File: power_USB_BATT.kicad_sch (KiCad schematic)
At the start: 17 parts, among them IC1 MCP73834T-FCI_UN, IC2 AP2112M-3.3TRG1, Q1 MCQ9435-TP

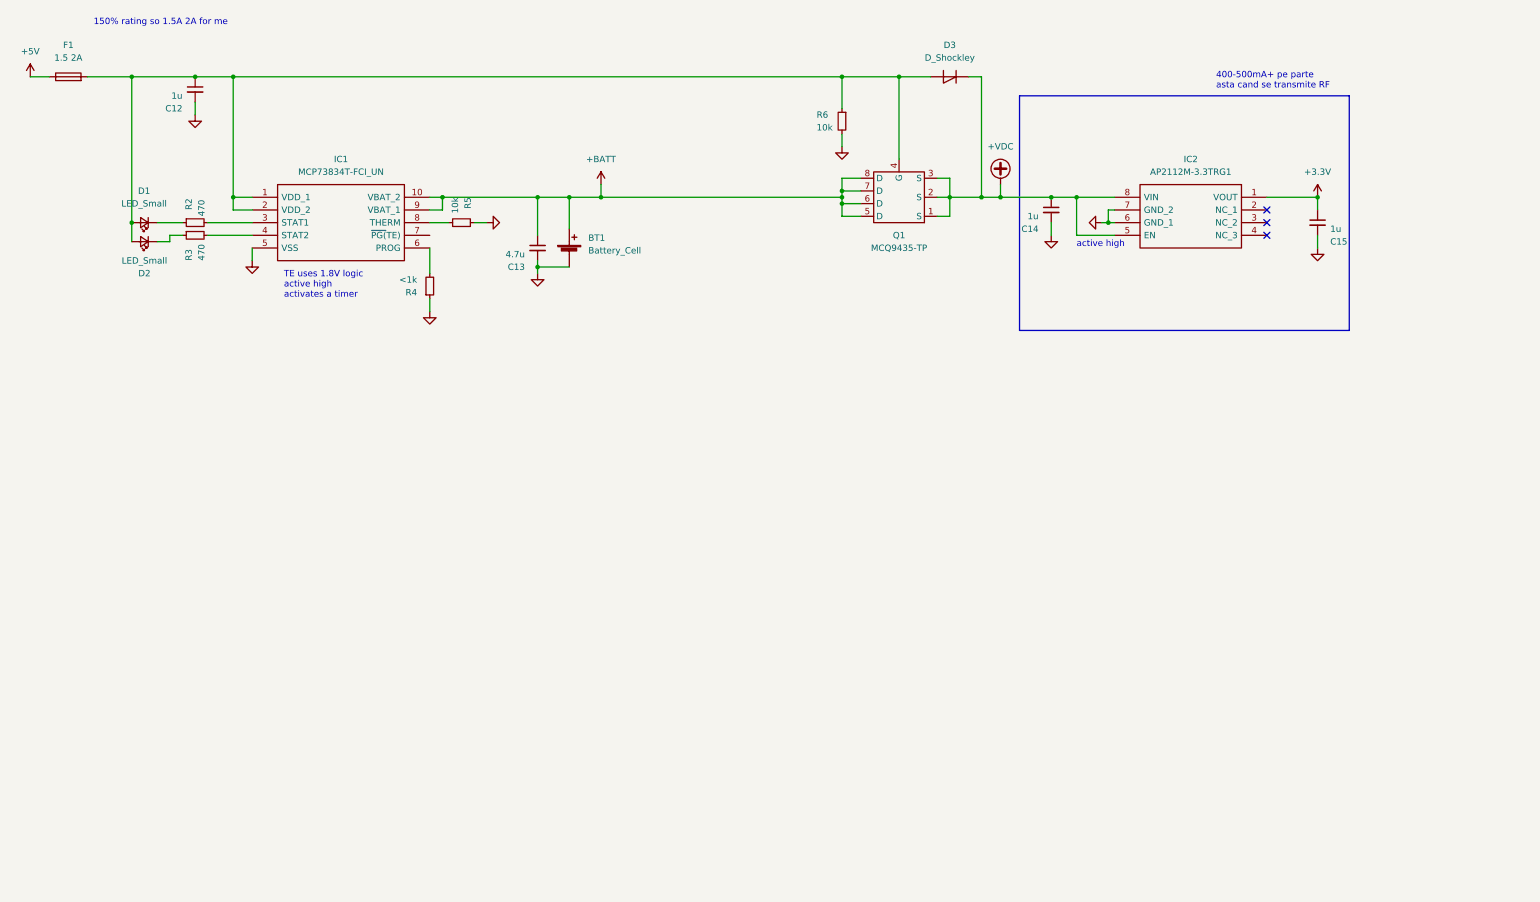
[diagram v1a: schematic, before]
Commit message: k
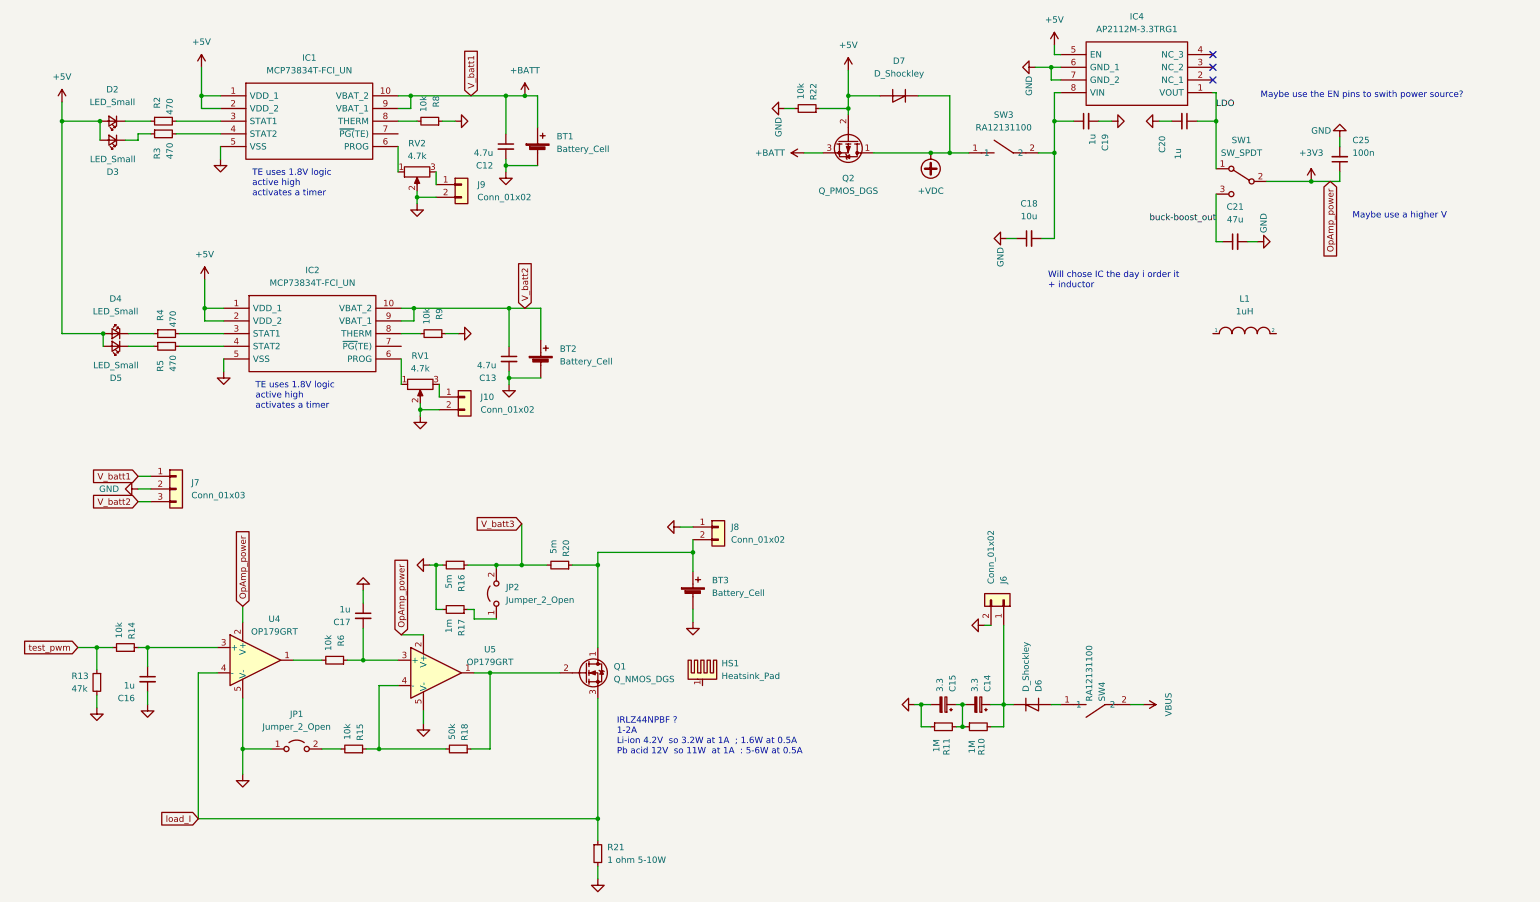
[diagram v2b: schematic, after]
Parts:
- removed C14, C15: 1u, symbol Device:C_Small
- removed D1: LED_Small, symbol Device:LED_Small
- removed D3: D_Shockley, Diode_THT:D_DO-15_P15.24mm_Horizontal, symbol Device:D_Shockley
- removed F1: 1.5 2A, symbol Device:Fuse
- removed IC2: AP2112M-3.3TRG1, SOIC127P600X170-8N, symbol SamacSys_Parts:AP2112M-3.3TRG1
- removed Q1: MCQ9435-TP, Package_SO:SOP-8_3.76x4.96mm_P1.27mm, symbol My_custom_lib:MCQ9435-TP
- added BT2, BT3: Battery_Cell, Connector_PinHeader_2.54mm:PinHeader_1x02_P2.54mm_Vertical, symbol Device:Battery_Cell
- added C14, C15: 3.3, Capacitor_THT:CP_Radial_D8.0mm_P3.50mm, symbol Device:C_Polarized_Small
- added C16, C17, C19, C20: 1u, Capacitor_SMD:C_0603_1608Metric_Pad1.08x0.95mm_HandSolder, symbol Device:C_Small
- added C18: 10u, symbol Device:C_Small
- added C21: 47u, symbol Device:C_Small
- added C25: 100n, Capacitor_SMD:C_0603_1608Metric_Pad1.08x0.95mm_HandSolder, symbol Device:C_Small
- added D3, D4, D5: LED_Small, LED_SMD:LED_0603_1608Metric_Pad1.05x0.95mm_HandSolder, symbol Device:LED_Small
- added D6, D7: D_Shockley, Diode_THT:D_A-405_P12.70mm_Horizontal, symbol Device:D_Shockley
- added HS1: Heatsink_Pad, symbol Mechanical:Heatsink_Pad
- added IC2: MCP73834T-FCI_UN, SamacSys_Parts:SOP50P490X110-10N, symbol SamacSys_Parts:MCP73834T-FCI_UN
- added IC4: AP2112M-3.3TRG1, SOIC127P600X170-8N, symbol SamacSys_Parts:AP2112M-3.3TRG1
- added J10, J9: Conn_01x02, Connector_PinHeader_2.54mm:PinHeader_1x02_P2.54mm_Vertical, symbol Connector_Generic:Conn_01x02
- added J6: Conn_01x02, Resistor_THT:R_Axial_DIN0309_L9.0mm_D3.2mm_P5.08mm_Vertical, symbol Connector_Generic:Conn_01x02
- added J7: Conn_01x03, Connector_PinHeader_2.54mm:PinHeader_1x03_P2.54mm_Vertical, symbol Connector_Generic:Conn_01x03
- added J8: Conn_01x02, Connector_Wago:Wago_734-132_1x02_P3.50mm_Vertical, symbol Connector_Generic:Conn_01x02
- added JP1, JP2: Jumper_2_Open, symbol Jumper:Jumper_2_Open
- added L1: 1uH, symbol pspice:INDUCTOR
- added Q1: Q_NMOS_DGS, symbol Device:Q_NMOS_DGS
- added Q2: Q_PMOS_DGS, symbol Device:Q_PMOS_DGS
- added R10, R11: 1M, Resistor_THT:R_Axial_DIN0411_L9.9mm_D3.6mm_P7.62mm_Vertical, symbol Device:R_Small
- added R13: 47k, Resistor_SMD:R_0603_1608Metric_Pad0.98x0.95mm_HandSolder, symbol Device:R_Small
- added R14, R15, R22, R8, R9: 10k, Resistor_SMD:R_0603_1608Metric_Pad0.98x0.95mm_HandSolder, symbol Device:R_Small
- added R16, R20: 5m, Resistor_SMD:R_0603_1608Metric_Pad0.98x0.95mm_HandSolder, symbol Device:R_Small
- added R17: 1m, Resistor_SMD:R_0603_1608Metric_Pad0.98x0.95mm_HandSolder, symbol Device:R_Small
- added R18: 50k, Resistor_SMD:R_0603_1608Metric_Pad0.98x0.95mm_HandSolder, symbol Device:R_Small
- added R21: 1 ohm 5-10W, symbol Device:R_Small
- added RV1, RV2: 4.7k, Z_mycustom_footprint_lib:2002102255, symbol Device:R_Potentiometer
- added SW1: SW_SPDT, symbol Switch:SW_SPDT
- added SW3, SW4: RA12131100, symbol My_custom_lib:RA12131100
- added U4, U5: OP179GRT, Package_TO_SOT_SMD:SOT-23-5, symbol Amplifier_Operational:OP179GRT
- BT1: footprint (none) -> Connector_PinHeader_2.54mm:PinHeader_1x02_P2.54mm_Vertical
- C12: value 1u -> 4.7u; footprint (none) -> Capacitor_SMD:C_0603_1608Metric_Pad1.08x0.95mm_HandSolder
- C13: footprint (none) -> Capacitor_SMD:C_0603_1608Metric_Pad1.08x0.95mm_HandSolder
- D2: footprint (none) -> LED_SMD:LED_0603_1608Metric_Pad1.05x0.95mm_HandSolder
- IC1: footprint SOP50P490X110-10N -> SamacSys_Parts:SOP50P490X110-10N
- R2, R3, R6: footprint (none) -> Resistor_SMD:R_0603_1608Metric_Pad0.98x0.95mm_HandSolder
- R4: value <1k -> 470; footprint (none) -> Resistor_SMD:R_0603_1608Metric_Pad0.98x0.95mm_HandSolder
- R5: value 10k -> 470; footprint (none) -> Resistor_SMD:R_0603_1608Metric_Pad0.98x0.95mm_HandSolder
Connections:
- net +3V3: now also C25.1, SW1.2 (B), U4.2 (V+), U5.2 (V+)
- net +5V: now also D2.2 (A), IC1.1 (VDD_1), IC1.2 (VDD_2), D3.2 (A), D4.2 (A), D5.2 (A), D7.2 (A), IC2.1 (VDD_1), IC2.2 (VDD_2), IC4.5 (EN), Q2.2 (G), R22.1
- net +BATT: now also C12.1, J7.1 (Pin_1), Q2.3 (S); no longer C13.1
- net +VDC: now also D7.1 (K), Q2.1 (D), SW3.1
- net GND: now also BT2.2 (-), BT3.2 (-), C15.2, C16.2, C17.1, C18.1, C19.2, C20.2, C21.2, C25.2, IC2.5 (VSS), IC4.6 (GND_1), IC4.7 (GND_2), J10.2 (Pin_2), J6.2 (Pin_2), J7.2 (Pin_2), J8.1 (Pin_1), J9.2 (Pin_2), JP1.1 (A), R11.1, R13.2, R16.2, R17.2, R21.2, R22.2, R8.1, R9.1, RV1.2, RV2.2, U4.5 (V-), U5.5 (V-); no longer R4.1, R5.1, R6.2
- net at R5.2: now also IC2.4 (STAT2); no longer IC1.8 (THERM)
- net at D2.1 (K): now also R2.1; no longer R3.1
- net at IC1.6 (PROG): now also RV2.1; no longer R4.2
- new net: C18.2, C19.1, IC4.8 (VIN), SW3.2
- new net: D5.1 (K), R5.1
- new net: J9.1 (Pin_1), RV2.3
- new net: IC2.8 (THERM), R9.2
- new net: J10.1 (Pin_1), RV1.3
- new net: D6.2 (A), SW4.1
- new net: BT3.1 (+), J8.2 (Pin_2), Q1.1 (D), R20.1
- new net: Q1.2 (G), R18.1, U5.1
- new net: R15.1, R18.2, U5.4 (-)
- new net: C14.2, C15.1, R10.1, R11.2
- new net: C17.2, R6.1, U5.3 (+)
- new net: R6.2, U4.1
- new net: JP2.1 (A), R17.1
- new net: JP1.2 (B), R15.2
- new net: C14.1, D6.1 (K), J6.1 (Pin_1), R10.2
- new net: D3.1 (K), R3.1
- new net: C16.1, R14.1, U4.3 (+)
- new net: IC1.8 (THERM), R8.2
- new net: D4.1 (K), R4.1
- new net: IC2.3 (STAT1), R4.2
- new net: IC2.6 (PROG), RV1.1
- new net LDO: C20.1, IC4.1 (VOUT), SW1.1 (A)
- new net VBUS: SW4.2
- new net V_batt2: BT2.1 (+), C13.1, IC2.10 (VBAT_2), IC2.9 (VBAT_1), J7.3 (Pin_3)
- new net V_batt3: JP2.2 (B), R16.1, R20.2
- new net buck-boost_out: C21.1, SW1.3 (C)
- new net load_I: Q1.3 (S), R21.1, U4.4 (-)
- new net test_pwm: R13.1, R14.2
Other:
- note added: "IRLZ44NPBF ? 1-2A Li-ion 4.2V so 3.2W at 1A ; 1.6W at 0.5A Pb acid 12V so 11W at 1A : 5-6W at 0.5A"
- note added: "Maybe use a higher V"
- note added: "Maybe use the EN pins to swith power source?"
- note added: "Will chose IC the day i order it + inductor"
- note removed: "150% rating so 1.5A 2A for me"
- note removed: "400-500mA+ pe parte asta cand se transmite RF"
- note removed: "active high"
